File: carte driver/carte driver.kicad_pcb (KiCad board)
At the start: 2 copper layers, 120 x 50 mm, 74 parts, among them J1 UART CP, J10 STEPPER 4, J11 STEPPER 3, J2 Conn_01x03, J3 UART BONUS, J4 Conn_01x02, J6 STEPPER G, J7 STEPPER D, J8 STEPPER 1, J9 STEPPER 2, SW2 SW_DIP_x02, SW3 SW_DIP_x02, SW4 SW_DIP_x02, SW5 SW_DIP_x02, SW6 SW_DIP_x02, SW7 SW_DIP_x02, U1 TMC2209_SILENTSTEPSTICK, U10 XIAO-HALF-HOLE-23P, U2 TMC2209_SILENTSTEPSTICK, U3 TMC2209_SILENTSTEPSTICK, U4 TMC2209_SILENTSTEPSTICK, U5 TMC2209_SILENTSTEPSTICK, U6 TMC2209_SILENTSTEPSTICK

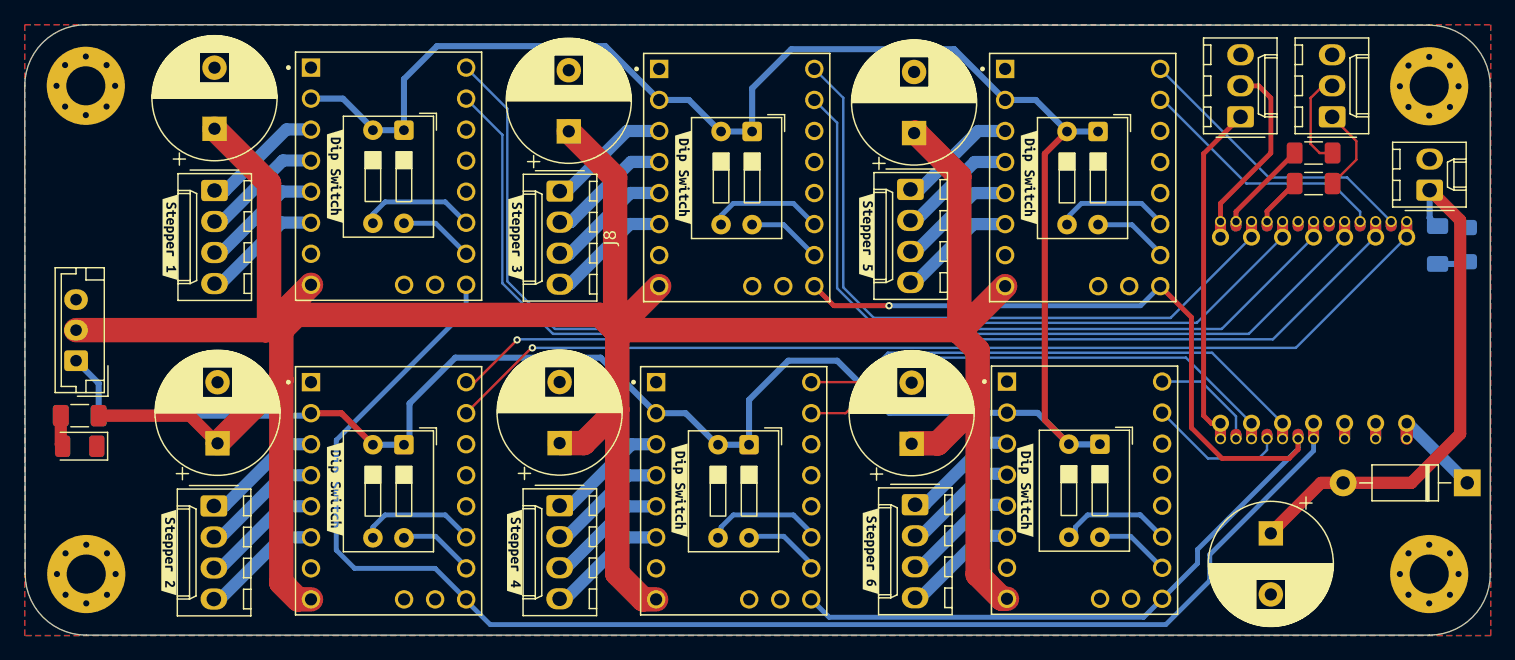
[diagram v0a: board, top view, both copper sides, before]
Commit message: caph
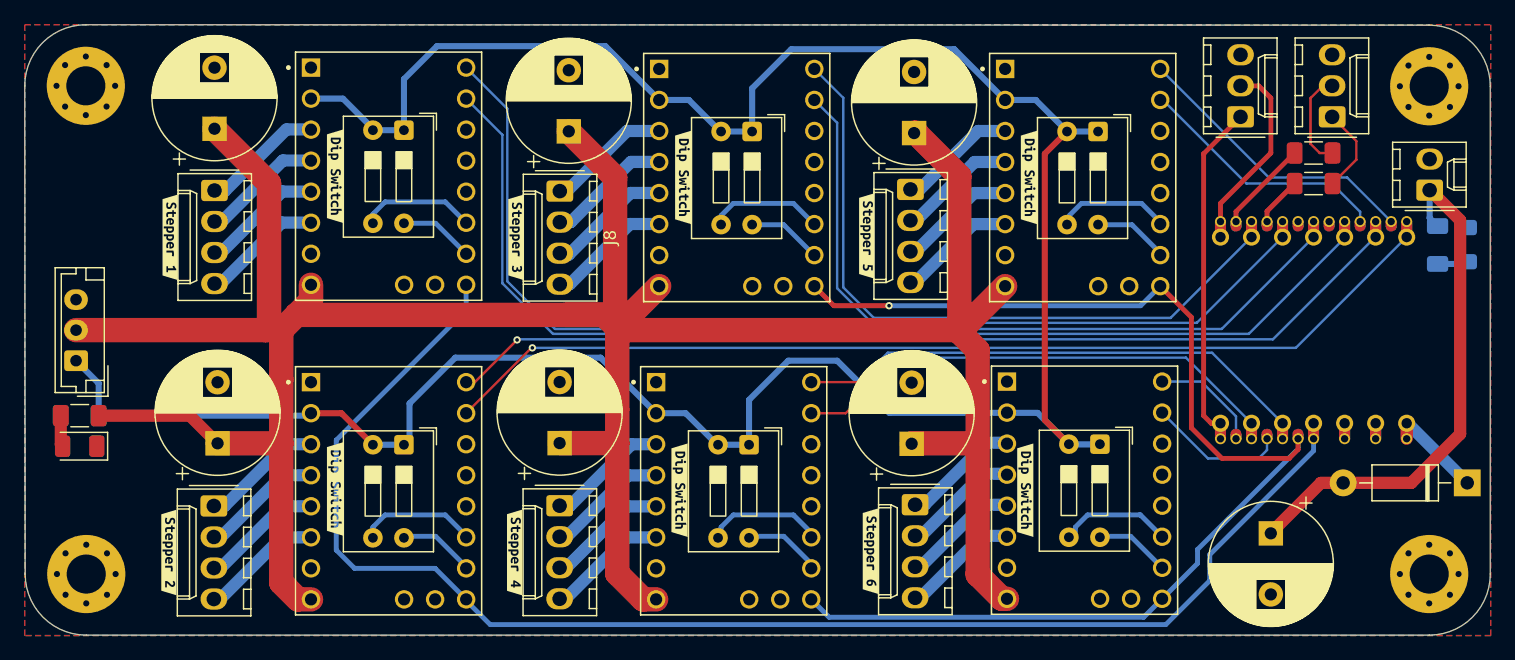
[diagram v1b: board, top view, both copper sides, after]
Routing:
- net +24V: track 247.7 -> 239.0 mm
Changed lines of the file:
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@@
 			(psa4output no)
 			(plot_black_and_white yes)
+			(plotinvisibletext no)
 			(sketchpadsonfab no)
 			(plotpadnumbers no)
@@
 	)
 	(segment
-		(start 105.4025 171.99)
-		(end 104.99 171.99)
+		(start 69.5325 133.725177)
+		(end 73.33 137.522677)
 		(width 2)
 		(layer "F.Cu")
@@
 	)
 	(segment
-		(start 104.99 171.99)
-		(end 103 170)
-		(width 2)
-		(layer "F.Cu")
-		(net 1)
-	)
-	(segment
 		(start 31.05 157)
 		(end 38.517322 157)
@@
 	)
 	(segment
-		(start 103 170)
-		(end 103 154.5)
+		(start 69.25 148.75)
+		(end 72.42 148.75)
 		(width 2)
 		(layer "F.Cu")
@@
 	)
 	(segment
-		(start 40.5325 133.515178)
-		(end 45 137.982678)
+		(start 73.5 156.5)
+		(end 73.5 150.17)
 		(width 2)
 		(layer "F.Cu")
@@
 	)
 	(segment
-		(start 68.7825 159.247678)
-		(end 70.752322 159.247678)
+		(start 97.63 159.27)
+		(end 102.98 159.27)
 		(width 2)
 		(layer "F.Cu")
@@
 	)
 	(segment
-		(start 73.5 150.17)
-		(end 73.33 150)
+		(start 73.08 148.75)
+		(end 47.25 148.75)
 		(width 2)
 		(layer "F.Cu")
@@
 	)
 	(segment
-		(start 101.5 150.1475)
-		(end 101.6475 150)
-		(width 2)
-		(layer "F.Cu")
-		(net 1)
-	)
-	(segment
-		(start 73.33 150)
-		(end 101.6475 150)
+		(start 45 137.982678)
+		(end 45 149)
 		(width 2)
 		(layer "F.Cu")
@@
 	)
 	(segment
-		(start 47.25 148.75)
-		(end 46 150)
+		(start 101.5 150.1475)
+		(end 101.5 137.4)
 		(width 2)
 		(layer "F.Cu")
@@
 	)
 	(segment
-		(start 97.6 159.3)
-		(end 97.63 159.27)
+		(start 104.99 171.99)
+		(end 103 170)
 		(width 2)
 		(layer "F.Cu")
@@
 	)
 	(segment
-		(start 97.8 133.867678)
-		(end 97.967678 133.867678)
+		(start 40.7825 159.265178)
+		(end 46 159.265178)
 		(width 2)
 		(layer "F.Cu")
@@
 	)
 	(segment
-		(start 76.9325 146.3975)
-		(end 73.33 150)
+		(start 73.67 150)
+		(end 101.6475 150)
 		(width 2)
 		(layer "F.Cu")
@@
 	)
 	(segment
-		(start 73.33 137.522677)
-		(end 73.33 150)
+		(start 97.967678 133.867678)
+		(end 97.8 133.867678)
 		(width 2)
 		(layer "F.Cu")
@@
 	)
 	(segment
-		(start 70.752322 159.247678)
-		(end 73.5 156.5)
+		(start 68.7825 159.247678)
+		(end 73.5 159.247678)
 		(width 2)
 		(layer "F.Cu")
@@
 	)
 	(segment
-		(start 45 149)
+		(start 47.25 148.75)
 		(end 46 150)
 		(width 2)
@@
 	)
 	(segment
-		(start 101.5 137.4)
-		(end 101.5 150.1475)
-		(width 2)
-		(layer "F.Cu")
-		(net 1)
-	)
-	(segment
-		(start 73.5 150.17)
-		(end 72.08 148.75)
+		(start 40.5325 133.515178)
+		(end 45 137.982678)
 		(width 2)
 		(layer "F.Cu")
@@
 	)
 	(segment
-		(start 69.5325 133.725177)
-		(end 73.33 137.522677)
+		(start 44.72 150)
+		(end 29.2 150)
 		(width 2)
 		(layer "F.Cu")
@@
 	)
 	(segment
-		(start 73.5 156.5)
-		(end 73.5 150.17)
+		(start 98 133.842855)
+		(end 97.824823 133.842855)
 		(width 2)
 		(layer "F.Cu")
@@
 	)
 	(segment
-		(start 97.63 159.27)
-		(end 99.73 159.27)
+		(start 102.98 159.27)
+		(end 103 159.25)
 		(width 2)
 		(layer "F.Cu")
@@
 	)
 	(segment
-		(start 44.72 150)
-		(end 29.2 150)
+		(start 46 170.671317)
+		(end 46 154.047678)
 		(width 2)
 		(layer "F.Cu")
@@
 	)
 	(segment
-		(start 45 137.982678)
-		(end 45 149)
+		(start 97.824823 133.842855)
+		(end 97.8 133.867678)
 		(width 2)
 		(layer "F.Cu")
@@
 	)
 	(segment
-		(start 98 133.842855)
-		(end 97.824823 133.842855)
+		(start 72.42 148.75)
+		(end 73.67 150)
 		(width 2)
 		(layer "F.Cu")
@@
 	)
 	(segment
-		(start 46 170.671317)
-		(end 46 154.047678)
+		(start 73.5 169.921317)
+		(end 73.5 156.5)
 		(width 2)
 		(layer "F.Cu")
@@
 	)
 	(segment
-		(start 97.824823 133.842855)
-		(end 97.8 133.867678)
+		(start 47.366183 172.0375)
+		(end 46 170.671317)
 		(width 2)
 		(layer "F.Cu")
@@
 	)
 	(segment
-		(start 73.5 169.921317)
-		(end 73.5 156.5)
+		(start 48.4325 147.5675)
+		(end 48.4325 146.2875)
 		(width 2)
 		(layer "F.Cu")
@@
 	)
 	(segment
-		(start 47.366183 172.0375)
-		(end 46 170.671317)
+		(start 97.6 159.3)
+		(end 97.63 159.27)
 		(width 2)
 		(layer "F.Cu")
@@
 	)
 	(segment
-		(start 40.7825 159.265178)
-		(end 46 154.047678)
+		(start 103 151.6475)
+		(end 101.5 150.1475)
 		(width 2)
 		(layer "F.Cu")
@@
 	)
 	(segment
-		(start 103 156)
-		(end 103 151.6475)
+		(start 101.5 137.4)
+		(end 97.967678 133.867678)
 		(width 2)
 		(layer "F.Cu")
@@
 	)
 	(segment
-		(start 72.08 148.75)
-		(end 47.25 148.75)
+		(start 48.4325 172.0375)
+		(end 47.366183 172.0375)
 		(width 2)
 		(layer "F.Cu")
@@
 	)
 	(segment
-		(start 48.4325 172.0375)
-		(end 47.366183 172.0375)
+		(start 103 170)
+		(end 103 151.6475)
 		(width 2)
 		(layer "F.Cu")
@@
 	)
 	(segment
-		(start 48.4325 146.2875)
-		(end 44.72 150)
+		(start 44.72 150)
+		(end 46 150)
 		(width 2)
 		(layer "F.Cu")
@@
 	)
 	(segment
-		(start 44.72 150)
-		(end 46 150)
+		(start 73.33 137.522677)
+		(end 73.33 148.5)
 		(width 2)
 		(layer "F.Cu")
@@
 	)
 	(segment
-		(start 97.967678 133.867678)
-		(end 101.5 137.4)
+		(start 73.67 149.66)
+		(end 76.9325 146.3975)
 		(width 2)
 		(layer "F.Cu")
@@
 	)
 	(segment
-		(start 99.73 159.27)
-		(end 103 156)
+		(start 47.25 148.75)
+		(end 48.4325 147.5675)
 		(width 2)
 		(layer "F.Cu")
@@
 	)
 	(segment
-		(start 103 151.6475)
-		(end 101.5 150.1475)
+		(start 105.4025 171.99)
+		(end 104.99 171.99)
 		(width 2)
 		(layer "F.Cu")
